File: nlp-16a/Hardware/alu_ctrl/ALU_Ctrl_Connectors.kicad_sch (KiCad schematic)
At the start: 85 parts, among them J1 Screw_Terminal_01x02, J10 Conn_02x08_Odd_Even, J2 Conn_02x20_Odd_Even, J3 Conn_02x10_Counter_Clockwise, J4 Conn_02x10_Counter_Clockwise, J5 Conn_02x10_Counter_Clockwise, J6 Conn_02x10_Counter_Clockwise, J7 Conn_02x10_Counter_Clockwise, J8 Conn_02x08_Odd_Even, J9 Conn_02x08_Odd_Even, U28 CD74HC00

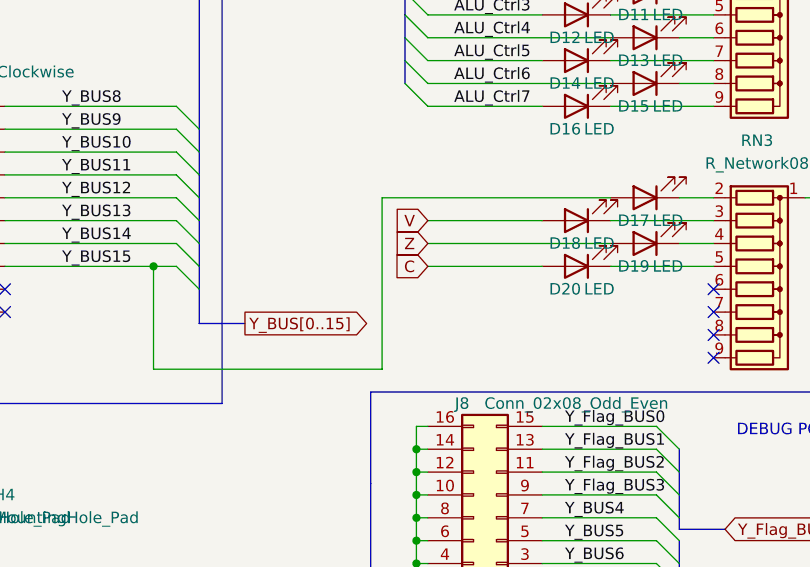
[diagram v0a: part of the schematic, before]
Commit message: だいたい完成．残りは詳細チェックとビア打ち
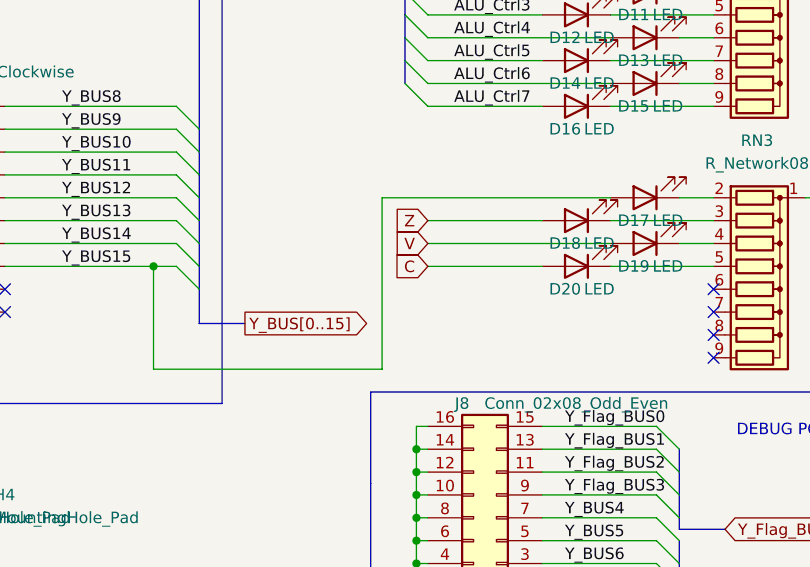
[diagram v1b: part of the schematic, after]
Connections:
- net V: now also D19.2 (A); no longer D18.2 (A)
- net Z: now also D18.2 (A); no longer D19.2 (A)
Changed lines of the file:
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@@
+    (stroke (width 0) (type default) (color 0 0 0 0))
+  )
+  (wire (pts (xy 147.32 86.36) (xy 160.02 86.36))
     (stroke (width 0) (type default) (color 0 0 0 0))
   )
@@
     (stroke (width 0) (type default) (color 0 0 0 0))
   )
+  (wire (pts (xy 142.24 78.74) (xy 167.64 78.74))
+    (stroke (width 0) (type default) (color 0 0 0 0))
+  )
   (wire (pts (xy 261.62 111.76) (xy 261.62 113.03))
     (stroke (width 0) (type default) (color 0 0 0 0))
@@
     (stroke (width 0) (type default) (color 0 0 0 0))
   )
-  (wire (pts (xy 147.32 86.36) (xy 160.02 86.36))
-    (stroke (width 0) (type default) (color 0 0 0 0))
-  )
   (wire (pts (xy 73.66 168.91) (xy 86.36 168.91))
     (stroke (width 0) (type default) (color 0 0 0 0))
@@
     (stroke (width 0) (type default) (color 0 0 0 0))
   )
-  (wire (pts (xy 142.24 78.74) (xy 167.64 78.74))
-    (stroke (width 0) (type default) (color 0 0 0 0))
-  )
   (wire (pts (xy 243.84 50.8) (xy 243.84 53.34))
     (stroke (width 0) (type default) (color 0 0 0 0))
@@
     (stroke (width 0) (type default) (color 0 0 0 0))
   )
-  (wire (pts (xy 142.24 97.79) (xy 142.24 78.74))
+  (wire (pts (xy 142.24 78.74) (xy 142.24 97.79))
     (stroke (width 0) (type default) (color 0 0 0 0))
   )
@@
     )
   )
-  (global_label "V" (shape input) (at 147.32 81.28 180) (fields_autoplaced)
+  (global_label "V" (shape input) (at 147.32 83.82 180) (fields_autoplaced)
     (effects (font (size 1.27 1.27)) (justify right))
-    (property "Intersheet References" "${INTERSHEET_REFS}" (id 0) (at 143.8183 81.2006 0)
+    (property "Intersheet References" "${INTERSHEET_REFS}" (id 0) (at 143.8183 83.7406 0)
       (effects (font (size 1.27 1.27)) (justify right) hide)
     )
@@
     )
   )
-  (global_label "Z" (shape input) (at 147.32 83.82 180) (fields_autoplaced)
+  (global_label "Z" (shape input) (at 147.32 81.28 180) (fields_autoplaced)
     (effects (font (size 1.27 1.27)) (justify right))
-    (property "Intersheet References" "${INTERSHEET_REFS}" (id 0) (at 143.6974 83.7406 0)
+    (property "Intersheet References" "${INTERSHEET_REFS}" (id 0) (at 143.6974 81.2006 0)
       (effects (font (size 1.27 1.27)) (justify right) hide)
     )
